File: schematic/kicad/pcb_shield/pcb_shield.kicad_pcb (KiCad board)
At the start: 2 copper layers, 70 x 57.5 mm, 9 parts, among them U2 NUCLEO-F411RE

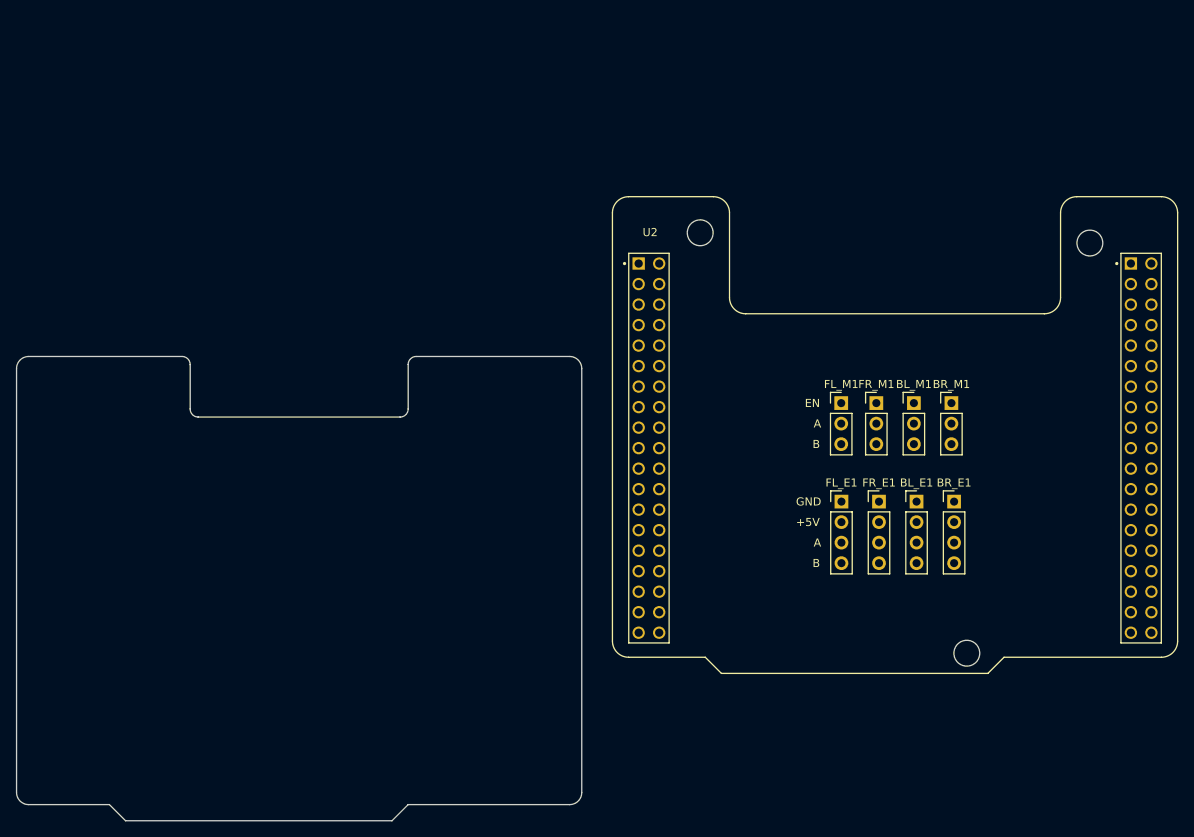
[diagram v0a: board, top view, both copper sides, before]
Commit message: change shield template1
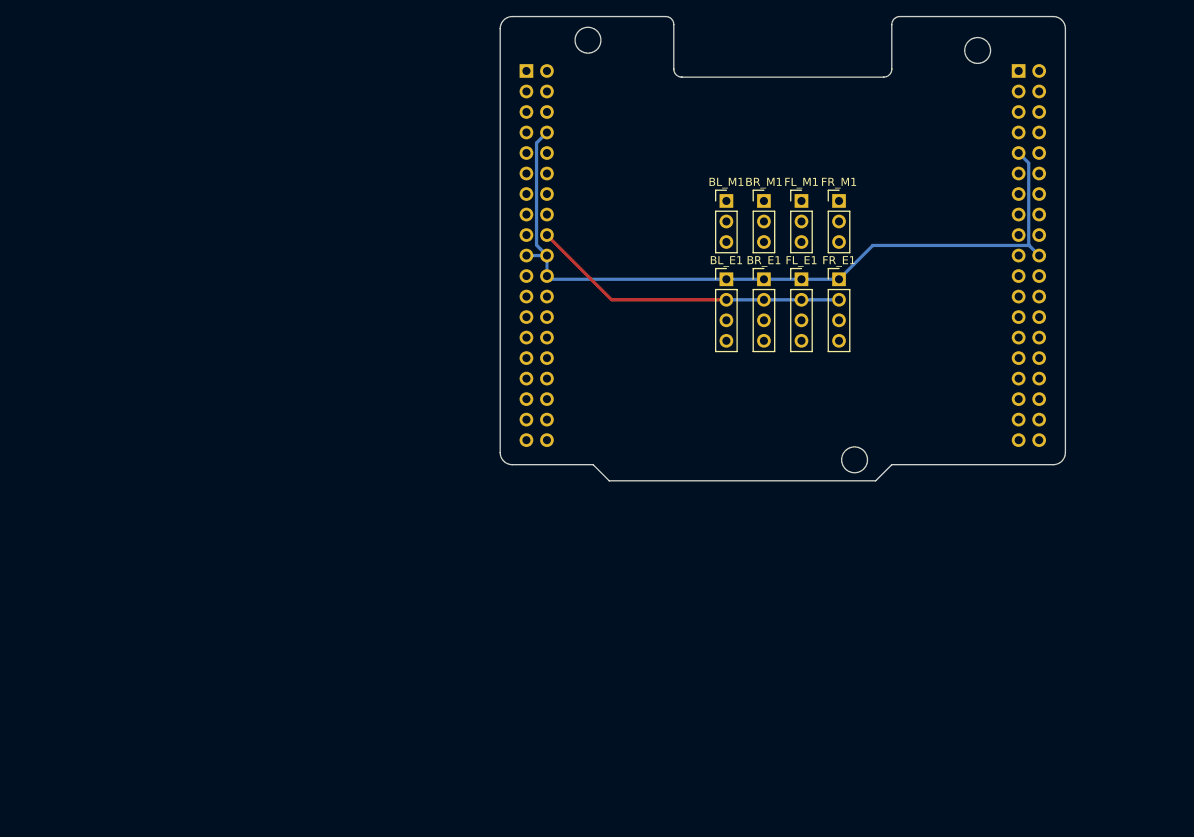
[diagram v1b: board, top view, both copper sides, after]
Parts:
- removed U2: NUCLEO-F411RE, NUCLEO-F411RE:BOARD_NUCLEO-F411RE_custom
- added H1: MountingHole, MountingHole:MountingHole_3.2mm_M3, F.Cu at (145.4, 110.4)
- added H2: MountingHole, MountingHole:MountingHole_3.2mm_M3, F.Cu at (112.4, 58.4)
- added H3: MountingHole, MountingHole:MountingHole_3.2mm_M3, F.Cu at (160.6, 59.7)
- added J1: CN7, Connector_PinSocket_2.54mm:PinSocket_2x19_P2.54mm_Vertical, B.Cu at (104.8, 62.2)
- added J2: CN10, Connector_PinSocket_2.54mm:PinSocket_2x19_P2.54mm_Vertical, B.Cu at (165.7, 62.2)
- moved BL_E1 36.2 mm to (129.5, 88.0)
- moved BR_E1 36.2 mm to (134.2, 88.0)
- moved BR_M1 34.1 mm to (134.2, 78.3)
- moved BL_M1 34.1 mm to (129.5, 78.3)
- moved FL_E1 28.0 mm to (138.8, 88.0)
- moved FR_E1 28.0 mm to (143.5, 88.0)
- moved FL_M1 25.5 mm to (138.8, 78.3)
- moved FR_M1 25.5 mm to (143.5, 78.3)
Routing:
- net GND: track 0.00 -> 96.8 mm
- net +5V: track 0.00 -> 39.5 mm
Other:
- board text removed: "+5V"
- board text removed: "A"
- board text removed: "B"
- board text removed: "EN"
- board text removed: "GND"
